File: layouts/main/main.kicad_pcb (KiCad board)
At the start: 4 copper layers, 20.5 x 20.5 mm, 60 parts

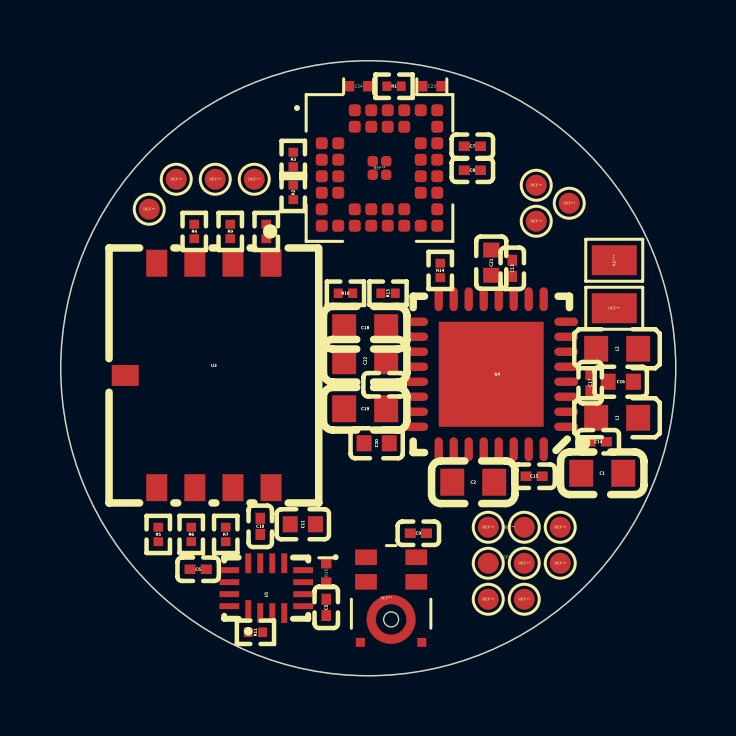
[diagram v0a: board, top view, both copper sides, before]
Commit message: wip
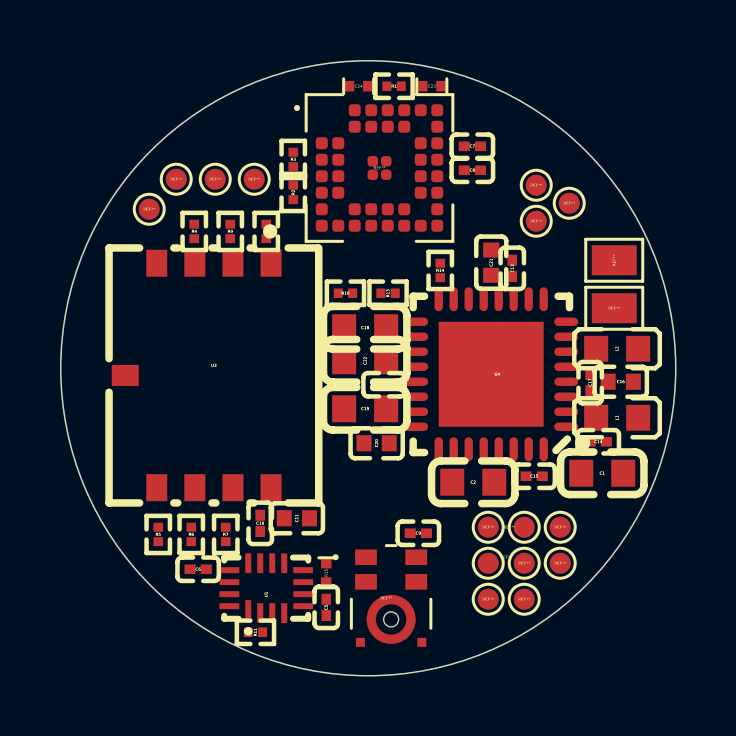
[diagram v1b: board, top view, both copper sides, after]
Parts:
- moved C11 0.28 mm to (-2.38, 5.00)
- moved C10 0.10 mm to (-3.60, 5.17)
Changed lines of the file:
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@@
 	(footprint "Murata_Electronics_GRM033R60J104KE19D:C0201"
 		(layer "F.Cu")
-		(at -3.6 5.27 -90)
+		(at -3.6 5.17 -90)
 		(property "Reference" "C10"
 			(at 0 -0.000167 0)
@@
 	(footprint "Samsung_Electro_Mechanics_CL05A225MQ5NSNC:C0402"
 		(layer "F.Cu")
-		(at -2.18 5.2)
+		(at -2.38 5)
 		(property "Reference" "C11"
 			(at 0 0 90)

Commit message: wip
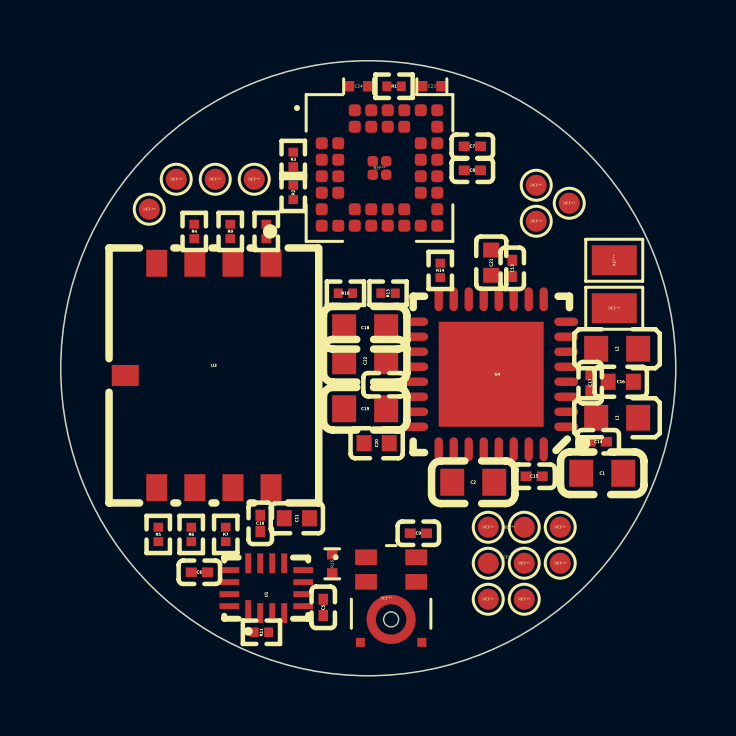
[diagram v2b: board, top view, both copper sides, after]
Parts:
- moved R15 0.36 mm to (-1.20, 6.52)
- moved R11 0.20 mm to (-3.56, 8.80)
- moved C6 0.11 mm to (-5.63, 6.80)
- moved C5 0.10 mm to (-1.50, 7.97)
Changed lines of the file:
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@@
 	(footprint "Murata_Electronics_GRM033R60J104KE19D:C0201"
 		(layer "F.Cu")
-		(at -5.67 6.7 180)
+		(at -5.63 6.8 180)
 		(property "Reference" "C6"
 			(at 0 -0.000166 0)
@@
 	(footprint "UNI_ROYAL_0201WMJ0330TEE:R0201"
 		(layer "F.Cu")
-		(at -3.76 8.8)
+		(at -3.56 8.8)
 		(property "Reference" "R11"
 			(at 0 0 90)
@@
 	(footprint "DNP_RES_0201:DNP_RES_0201"
 		(layer "F.Cu")
-		(at -1.4 6.82 -90)
+		(at -1.2 6.52 -90)
 		(property "Reference" "R15"
 			(at 0 0 90)
@@
 	(footprint "Murata_Electronics_GRM033R60J104KE19D:C0201"
 		(layer "F.Cu")
-		(at -1.4 7.97 -90)
+		(at -1.5 7.97 -90)
 		(property "Reference" "C5"
 			(at 0 -0.000167 90)
